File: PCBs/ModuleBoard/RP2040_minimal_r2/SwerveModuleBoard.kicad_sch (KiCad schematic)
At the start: 60 parts, among them IC1 AS5600-ASOT, J1 USB_B_Micro, J3 Conn_02x08_Odd_Even_MountingP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, J4 Conn_01x07, J5 Conn_01x06_Pin, J6 Conn_01x02, J7 Conn_01x06_Pin, J8 Conn_01x06, U1 NCP1117-3.3_SOT223, U2 W25Q128JVS, U3 RP2040, U4 DRV8245HQRXZRQ1, U5 DRV8245HQRXZRQ1, U7 TPS63051RMWR, Y1 ABM8-272-T3

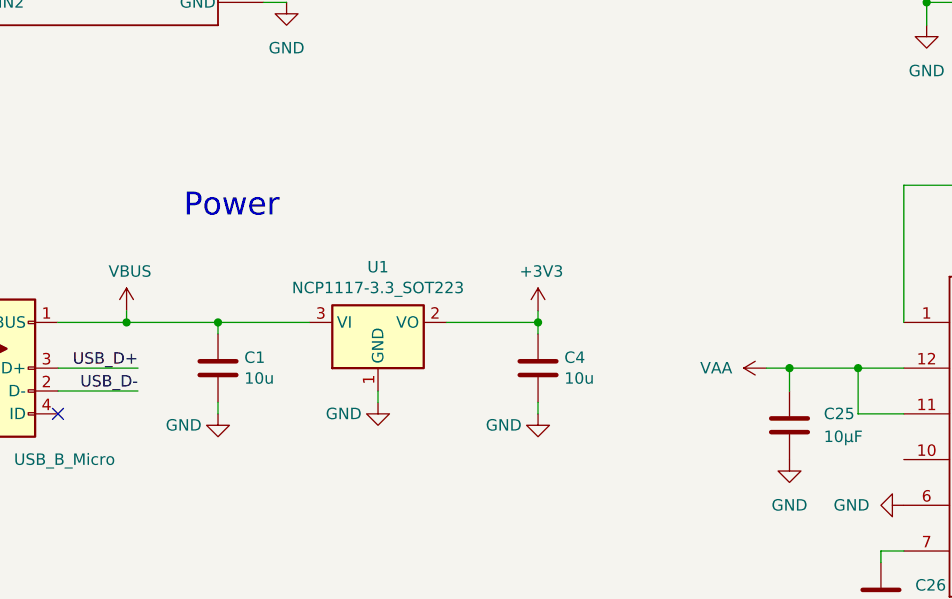
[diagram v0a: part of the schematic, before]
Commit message: vault backup: 2025-04-24 19:34:02
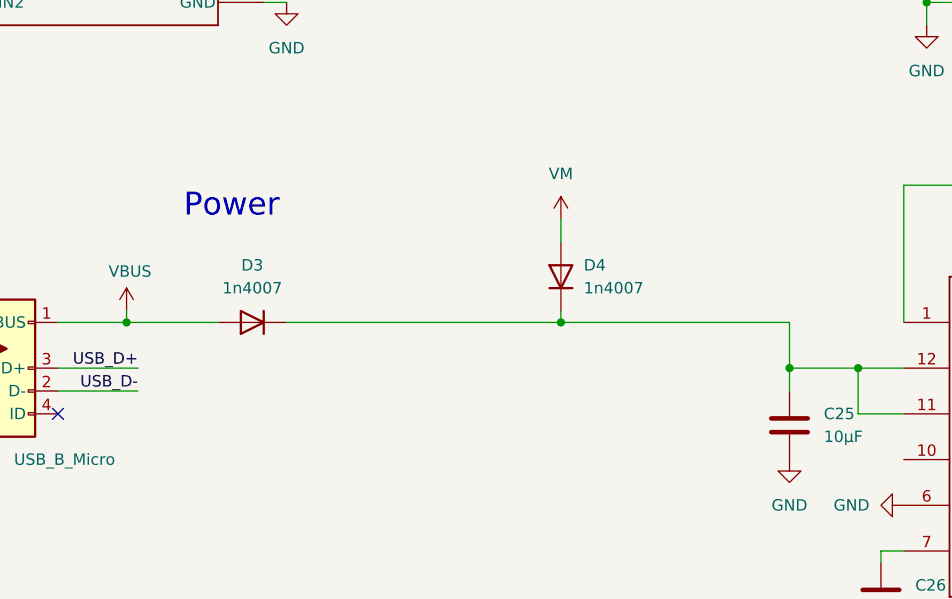
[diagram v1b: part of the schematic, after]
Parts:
- removed C1, C4: 10u, Capacitor_SMD:C_0603_1608Metric_Pad1.08x0.95mm_HandSolder, symbol Device:C
- removed U1: NCP1117-3.3_SOT223, Package_TO_SOT_SMD:SOT-223-3_TabPin2, symbol Regulator_Linear:NCP1117-3.3_SOT223
- added D3, D4: 1n4007, symbol Device:D
- U7: footprint RMW0012A -> BuckBoost:QFN50P250X250X100-12N
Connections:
- net VBUS: now also D3.2 (A)
- net VM: now also D4.2 (A)
- net VAA: no longer names the net of C25.1, U7.11 (EN), U7.12 (VIN)
- net VAA: now also D3.1 (K), D4.1 (K)

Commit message: vault backup: 2025-04-24 19:44:10
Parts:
- D3, D4: footprint (none) -> Diode_SMD:D_SOD-123
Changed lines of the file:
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@@
 			)
 		)
-		(property "Footprint" ""
+		(property "Footprint" "Diode_SMD:D_SOD-123"
 			(at 137.16 285.75 0)
 			(effects
@@
 			)
 		)
-		(property "Footprint" ""
+		(property "Footprint" "Diode_SMD:D_SOD-123"
 			(at 102.87 290.83 0)
 			(effects
